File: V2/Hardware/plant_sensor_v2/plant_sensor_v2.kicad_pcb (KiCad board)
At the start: 2 copper layers, 28.6 x 28.6 mm, 45 parts, among them IC1 ICM-20948, J1 TC2030_SWD-MCP-NL, U1 STM32WBA52KGUx, U2 TPS22960RSER, U3 TPS62840DLCR, Y1 32.768kHz, Y2 32MHz

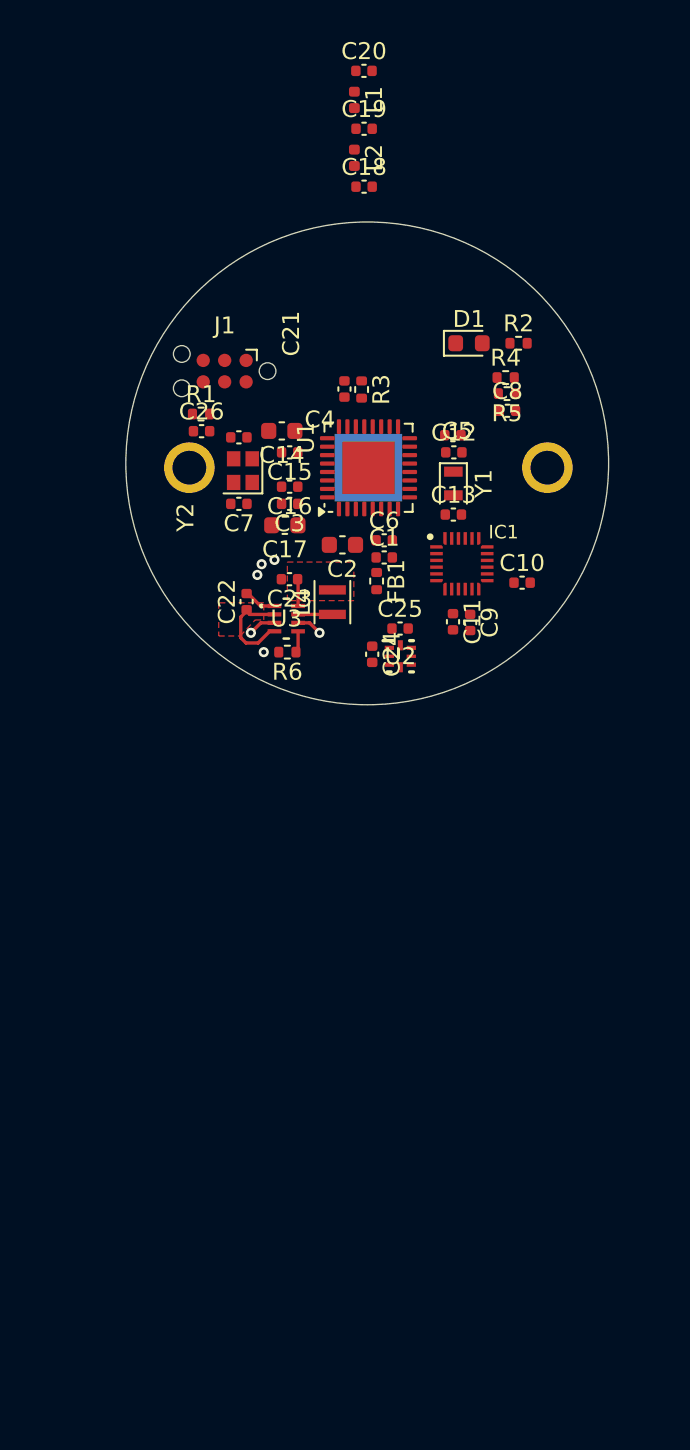
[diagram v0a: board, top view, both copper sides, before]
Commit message: update hardware
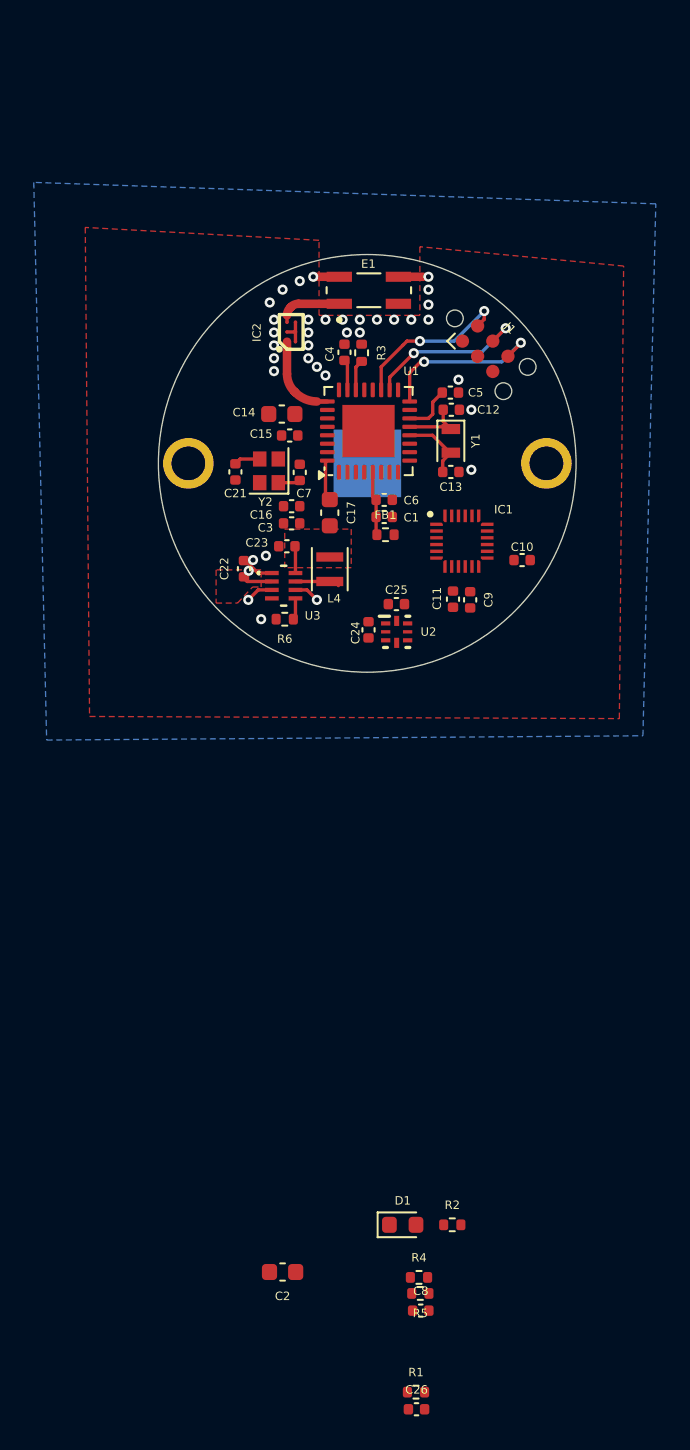
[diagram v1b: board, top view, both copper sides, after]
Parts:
- removed C18: 1.5p, Capacitor_SMD:C_0402_1005Metric
- removed C19: 3.9p, Capacitor_SMD:C_0402_1005Metric
- removed C20: 2.7p, Capacitor_SMD:C_0402_1005Metric
- removed L1: 1.3n, Inductor_SMD:L_0402_1005Metric
- removed L2: 1.8n, Inductor_SMD:L_0402_1005Metric
- added E1: 609-2450AT42E0100001, Antenna:XDCR_2450AT42E0100E, F.Cu at (102.9, 61.5)
- added IC2: MLPF-WB-04D3, MLPF-WB-04D3:BGA6C50P3X2_160X100X68, F.Cu at (98.3, 64.0)
- moved C26 59.3 mm to (105.7, 127.8)
- moved R1 59.3 mm to (105.7, 126.7)
- moved C8 53.5 mm to (106.0, 121.9)
- moved R4 53.5 mm to (105.9, 120.0)
- moved R5 53.5 mm to (105.9, 120.9)
- moved D1 52.3 mm to (104.9, 116.8)
- moved R2 52.3 mm to (107.8, 116.8)
- moved C2 43.2 mm to (97.8, 119.6)
- moved J1 15.5 mm to (109.8, 65.0), turned to -45 degrees
- moved C7 4.06 mm to (98.8, 72.3), turned to 90 degrees
- moved FB1 2.80 mm to (103.9, 76.0), turned to 0 degrees
- moved C17 2.76 mm to (100.6, 74.7), turned to -90 degrees
- moved C5 2.53 mm to (107.7, 67.6)
- moved C12 2.53 mm to (107.8, 68.6)
- moved C13 2.53 mm to (107.8, 72.3)
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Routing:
- net /SWO: track 0.00 -> 10.4 mm, vias 0 -> 2
- net /SWCLK: track 0.00 -> 9.90 mm, vias 0 -> 2
- net /SWDIO: track 0.00 -> 9.87 mm, vias 0 -> 2
- net /RF: track 0.00 -> 5.17 mm
- net +1V8: track 1.64 -> 6.43 mm
- net GND: track 5.15 -> 9.83 mm, vias 6 -> 36
- net /CRYSTAL2: track 0.00 -> 4.20 mm
- net Net-(IC2-OUT): track 0.00 -> 4.13 mm
- net +BATT: track 5.85 -> 1.73 mm
- net /CRYSTAL1: track 0.00 -> 3.82 mm
- net Net-(U1-VDDA): track 0.00 -> 3.80 mm
- net Net-(U1-VCAP): track 0.00 -> 2.46 mm
- net Net-(U1-PH3): track 0.00 -> 1.83 mm
- net /OSC_OUT: track 0.00 -> 1.56 mm
- net /OSC_IN: track 0.00 -> 1.32 mm
- added copper zone on B.Cu, net GND
- added copper zone on F.Cu, net GND
- added copper zone on In1.Cu, net GND
- added copper zone on In2.Cu, net GND
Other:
- board size 28.6 x 28.6 mm -> 24.7 x 24.7 mm
- copper layers 2 -> 4
